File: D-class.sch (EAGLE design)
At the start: 73 parts, among them IC1 TPA3118D2, IC2 7812, IC3 78L12

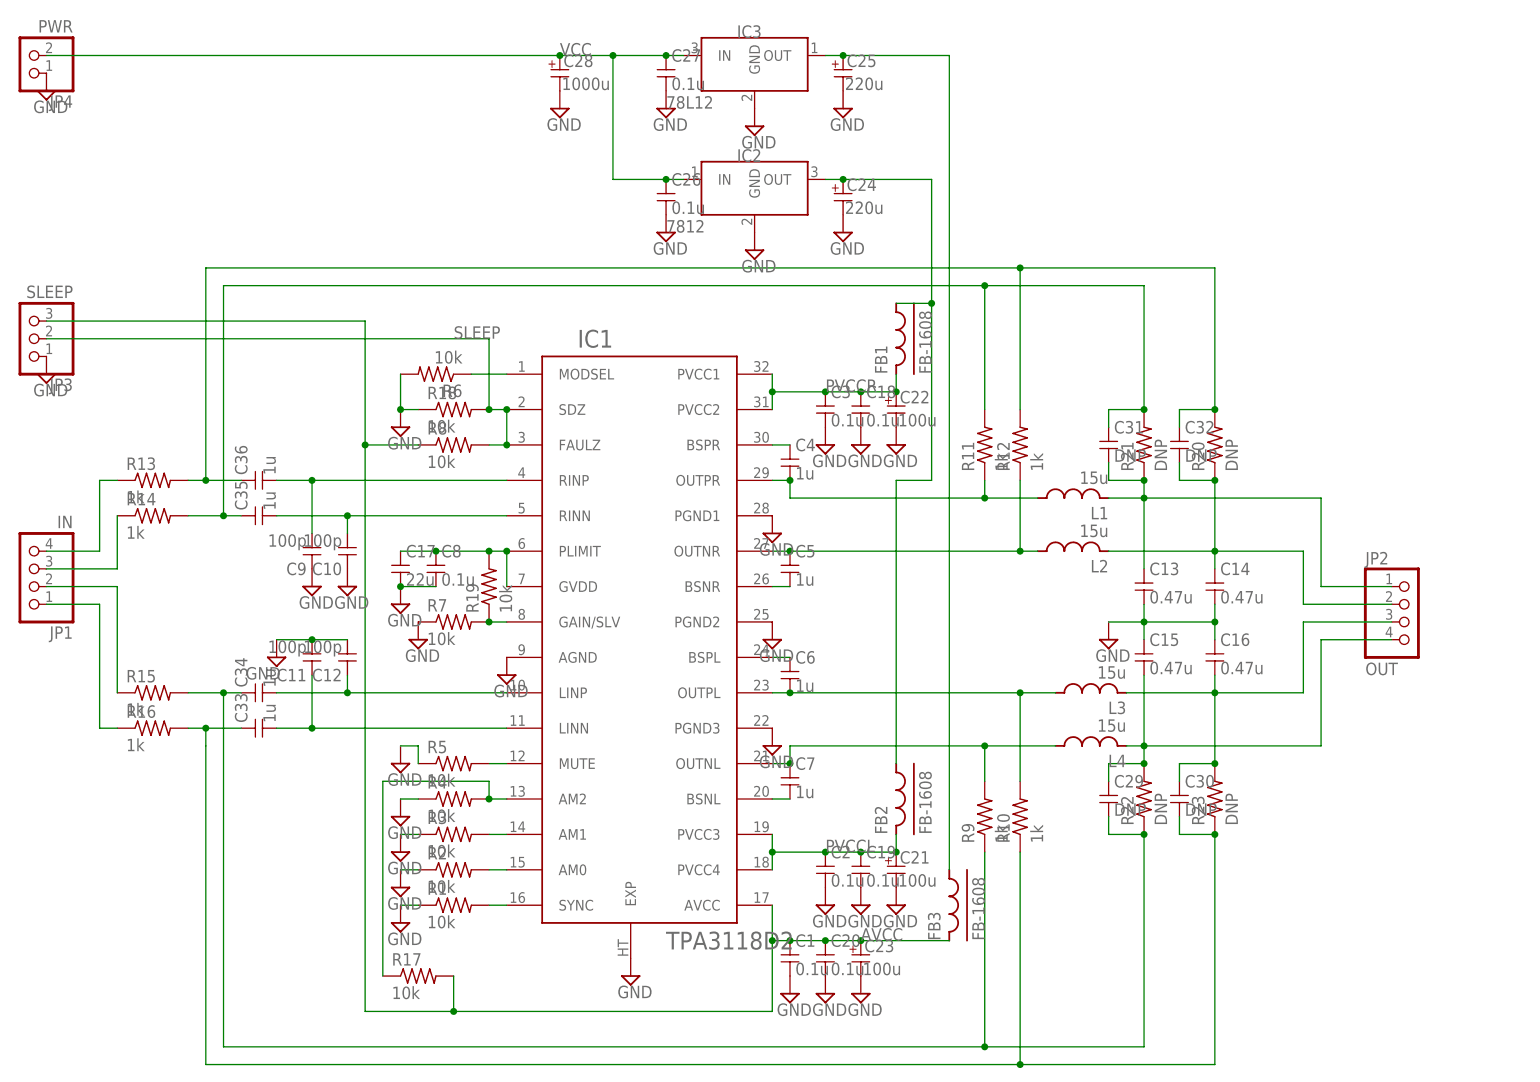
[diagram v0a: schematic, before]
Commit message: 後はGNDのみ
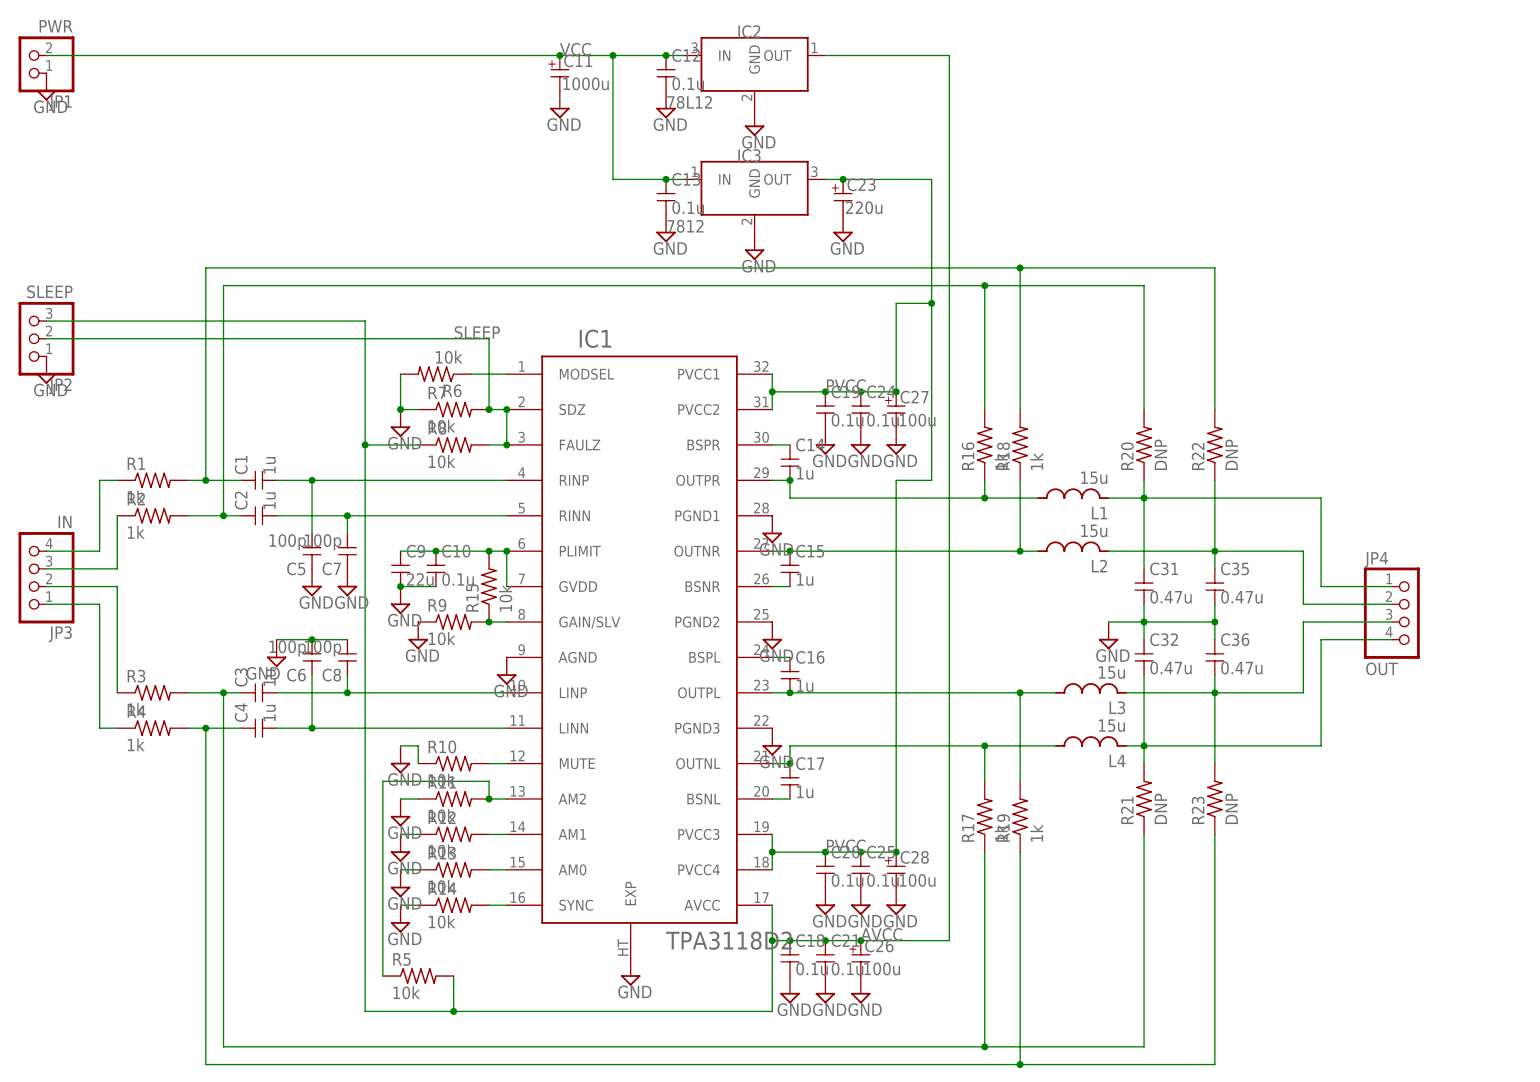
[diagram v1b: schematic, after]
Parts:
- removed C22: 100u, my_rcl:CPOLE2.5-6.5
- removed C29, C30: DNP, my_rcl:C-1608
- removed C33, C34: 1u, my_rcl:C-3216
- removed FB1, FB2, FB3: FB-1608, my_rcl:FB-1608
- C1, C2, C3: value 0.1u -> 1u; device my_rcl:C-1608 -> my_rcl:C-3216
- C10, C12: value 100p -> 0.1u
- C11: value 100p -> 1000u; device my_rcl:C-1608 -> my_rcl:CPOLE2.5-8
- C13: value 0.47u -> 0.1u; device my_rcl:C-5 -> my_rcl:C-1608
- C14, C15, C16: value 0.47u -> 1u; device my_rcl:C-5 -> my_rcl:C-1608
- C17: value 22u -> 1u; device my_rcl:C-2012 -> my_rcl:C-1608
- C18, C19, C20: device my_rcl:C-2012 -> my_rcl:C-1608
- C21: value 100u -> 0.1u; device my_rcl:CPOLE2.5-6.5 -> my_rcl:C-2012
- C23: value 100u -> 220u; device my_rcl:CPOLE2.5-6.5 -> my_rcl:CPOLE2.5-8
- C24, C25: value 220u -> 0.1u; device my_rcl:CPOLE2.5-8 -> my_rcl:C-2012
- C26, C27: value 0.1u -> 100u; device my_rcl:C-1608 -> my_rcl:CPOLE2.5-6.5
- C28: value 1000u -> 100u; device my_rcl:CPOLE2.5-8 -> my_rcl:CPOLE2.5-6.5
- C31, C32: value DNP -> 0.47u; device my_rcl:C-1608 -> my_rcl:C-5
- C35, C36: value 1u -> 0.47u; device my_rcl:C-3216 -> my_rcl:C-5
- C4: device my_rcl:C-1608 -> my_rcl:C-3216
- C5, C6, C7: value 1u -> 100p
- C8: value 0.1u -> 100p
- C9: value 100p -> 22u; device my_rcl:C-1608 -> my_rcl:C-2012
- IC2: value 7812 -> 78L12; device my_ic:78X-2 -> my_ic:78LX
- IC3: value 78L12 -> 7812; device my_ic:78LX -> my_ic:78X-2
- JP1: value IN -> PWR; device pinhead:PINHD-1X4 -> pinhead:PINHD-1X2
- JP2: value OUT -> SLEEP; device pinhead:PINHD-1X4 -> pinhead:PINHD-1X3
- JP3: value SLEEP -> IN; device pinhead:PINHD-1X3 -> pinhead:PINHD-1X4
- JP4: value PWR -> OUT; device pinhead:PINHD-1X2 -> pinhead:PINHD-1X4
- R1, R17, R18, R19, R2, R3, R4: value 10k -> 1k; device my_rcl:R-1608 -> my_rcl:R-2.5
- R10, R11, R12, R13, R14, R15, R9: value 1k -> 10k; device my_rcl:R-2.5 -> my_rcl:R-1608
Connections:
- removed net N$33: C24.1, FB1.1, FB2.1, IC2.OUT
- removed net PVCCL: C19.1, C2.1, C21.1, FB2.2, IC1.PVCC3, IC1.PVCC4
- removed net PVCCR: C18.1, C22.1, C3.1, FB1.2, IC1.PVCC1, IC1.PVCC2
- net AVCC: now also C18.1, C21.1, C26.1, IC2.OUT, JP2.3, R5.2; no longer C1.1, C20.1, C23.1, FB3.2, JP3.3, R17.2
- net GND: now also C10.2, C31.2, C32.1, C35.2, C36.1, C5.1, C6.2, C7.1, C9.2, JP1.1, JP2.1, R10.1, R11.1, R12.1, R13.1, R14.1, R9.1; no longer C1.2, C10.1, C14.2, C15.1, C16.1, C17.2, C2.2, C22.2, C3.2, C9.1, JP3.1, JP4.1, R1.1, R18.1, R2.1, R3.1, R4.1, R5.1
- net N$1: now also C2.2, C7.2; no longer C10.2, C35.2
- net N$10: now also C16.2, R19.2; no longer C6.2, R10.2
- net N$11: now also C16.1; no longer C6.1
- net N$12: now also C15.2; no longer C5.2
- net N$13: now also C15.1, R18.1; no longer C5.1, R12.1
- net N$14: now also C14.2, R16.1; no longer C4.2, R11.1
- net N$15: now also C14.1; no longer C4.1
- net N$18: now also C3.2, C8.1; no longer C12.1, C34.2
- net N$19: now also C10.1, C9.1, R15.2; no longer C17.1, C8.1, R19.2
- net N$2: now also R11.2, R5.1; no longer R17.1, R4.2
- net N$20: now also R15.1, R9.2; no longer R19.1, R7.2
- net N$21: now also C3.1, R17.1, R21.1, R3.2; no longer C29.2, C34.1, R15.2, R22.1, R9.1
- net N$22: now also C4.1, R19.1, R4.2; no longer C30.2, C33.1, R10.1, R16.2
- net N$23: now also C1.1, R1.2, R18.2, R22.2; no longer C32.1, C36.1, R12.2, R13.2, R20.2
- net N$24: now also C2.1, R16.2, R2.2, R20.2; no longer C31.1, C35.1, R11.2, R14.2, R21.2
- net N$25: now also C36.2, JP4.3; no longer C16.2, C30.1, JP2.3
- net N$26: now also C32.2, JP4.4, R21.2; no longer C15.2, C29.1, JP2.4, R22.2
- net N$27: now also C35.1, JP4.2, R22.1; no longer C14.1, C32.2, JP2.2, R20.1
- net N$28: now also C31.1, JP4.1, R20.1; no longer C13.1, C31.2, JP2.1, R21.1
- net N$29: now also JP3.2, R3.1; no longer JP1.2, R15.1
- net N$3: now also R12.2; no longer R3.2
- net N$30: now also JP3.1, R4.1; no longer JP1.1, R16.1
- net N$31: now also JP3.3, R2.1; no longer JP1.3, R14.1
- net N$32: now also JP3.4, R1.1; no longer JP1.4, R13.1
- net N$37: now also R10.2; no longer R5.2
- net N$38: now also C1.2, C5.2; no longer C36.2, C9.2
- net N$39: now also C4.2, C6.1; no longer C11.1, C33.2
- net N$4: now also R13.2; no longer R2.2
- net N$5: now also R14.2; no longer R1.2
- net N$8: now also C17.2; no longer C7.2
- net N$9: now also C17.1, R17.2; no longer C7.1, R9.2
- net PVCC: now also C19.1, C20.1, C23.1, C24.1, C27.1, C28.1, IC1.PVCC1, IC1.PVCC2, IC1.PVCC3, IC1.PVCC4; no longer FB3.1
- net SLEEP: now also JP2.2, R7.2; no longer JP3.2, R18.2
- net VCC: now also C11.1, C12.1, C13.1, JP1.2; no longer C26.1, C27.1, C28.1, JP4.2
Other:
- moved on the sheet: C1, C10, C12, C13, C14, C15, C16, C17, C18, C19, C2, C20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

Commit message: 後はシルクのみ
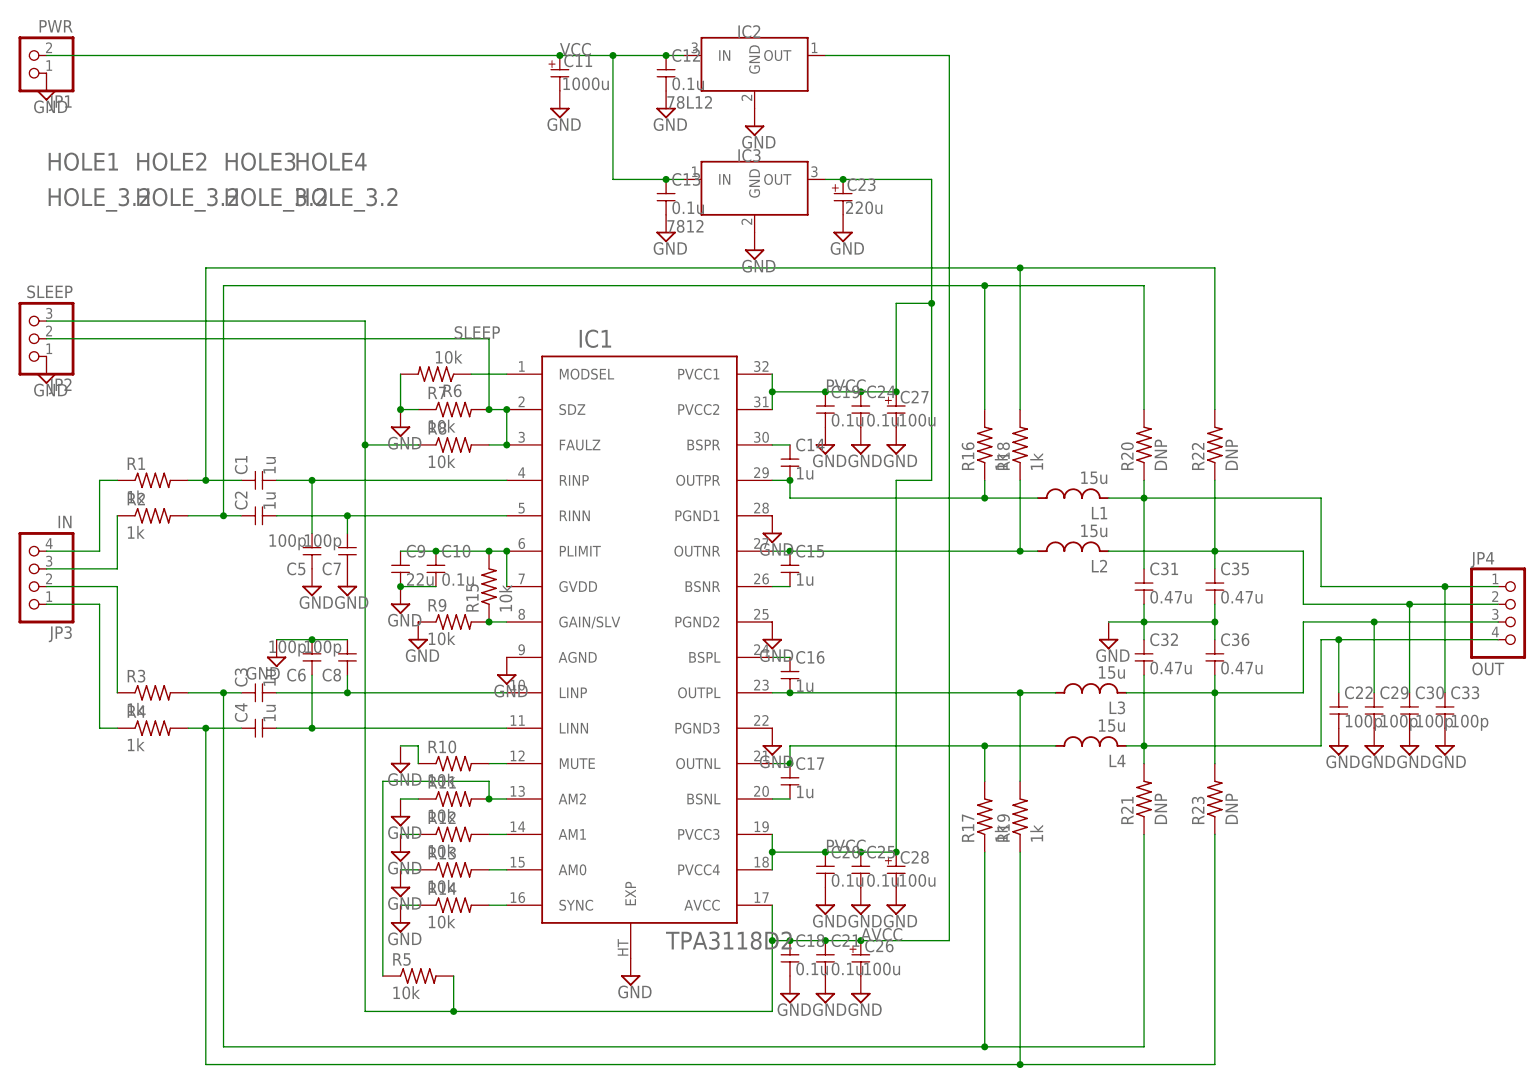
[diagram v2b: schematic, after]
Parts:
- added C22, C29, C30, C33: 100p, my_rcl:C-1608
- added HOLE1, HOLE2, HOLE3, HOLE4: HOLE_3.2, Document_Robotech:HOLE_3.2
- C11, C23: device my_rcl:CPOLE2.5-8 -> my_rcl:CPOLE5-10
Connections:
- net GND: now also C22.2, C29.2, C30.2, C33.2
- net N$25: now also C29.1
- net N$26: now also C22.1
- net N$27: now also C30.1
- net N$28: now also C33.1
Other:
- moved on the sheet: JP4
